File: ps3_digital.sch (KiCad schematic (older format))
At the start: 78 parts, among them SW2 SW_SPST, U1 SN75107B, U10 74LS08, U11 7425, U12 74LS32, U13 74LS193, U14 74LS153, U15 74LS74, U16 74LS93, U17 74LS244, U18 74LS367, U19 74LS367, U2 74LS175, U20 74LS32, U21 74LS74, U22 74LS266, U23 74LS266, U25 74LS08, U26 74LS08, U27 CD4051B, U28 74LS259, U29 74LS13, U3 74LS74, U30 74LS93, U31 74LS93, U32 74LS93, U33 74LS42, U34 74LS32, U35 74LS04, U36 7404, U37 4041, U38 4041, U39 TL072, U4 D2102, U40 TL082, U41 TL082, U42 TL082, U43 TL082, U44 L7805, U5 74LS00, U6 74LS04, U7 74LS10, U8 74LS00, U9 74LS32

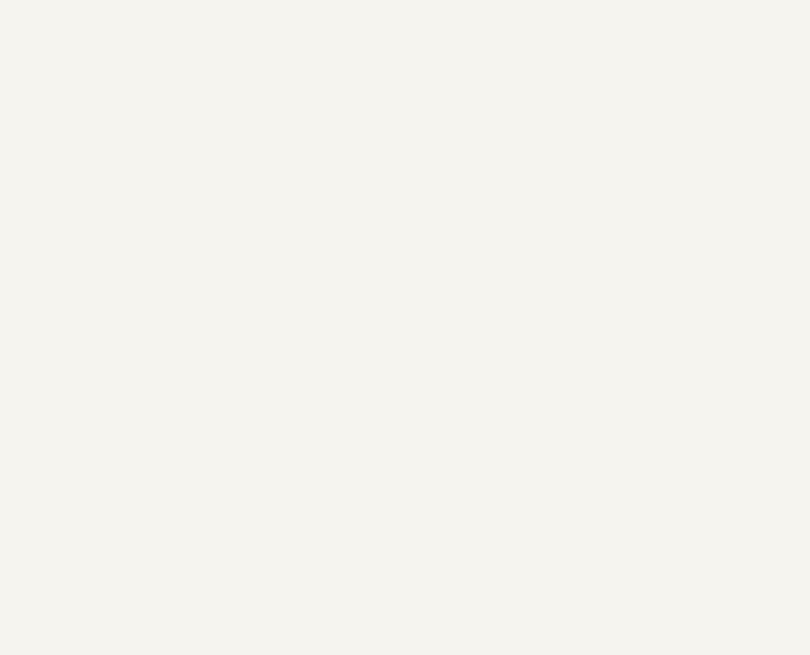
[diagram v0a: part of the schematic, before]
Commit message: 6810
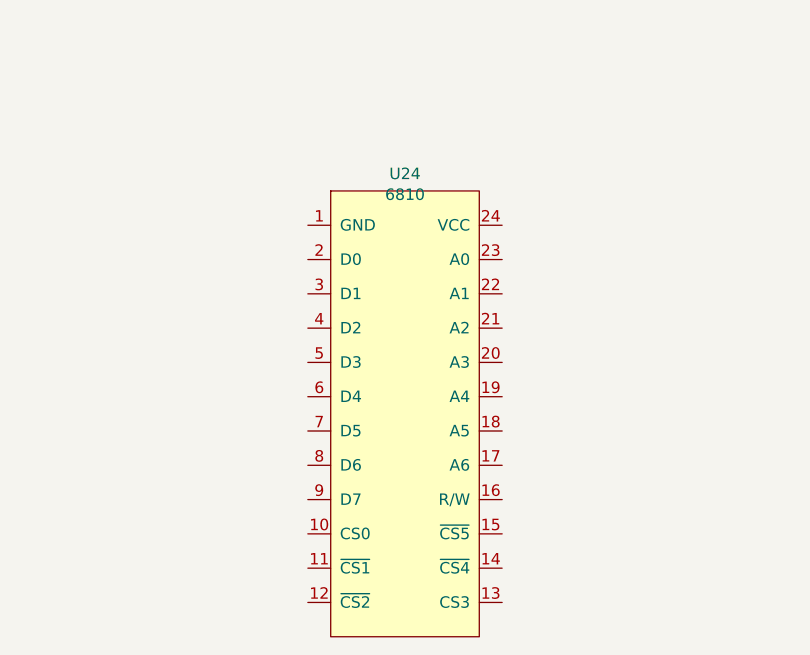
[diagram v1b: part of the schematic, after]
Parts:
- added U24: 6810, Package_DIP:DIP-24_W10.16mm_LongPads, symbol Memory_RAM:6810
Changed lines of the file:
@@
 	20250 6600 20500 6600
 Connection ~ 20250 6600
+$Comp
+L Memory_RAM:6810 U24
+U 1 1 5F25EB04
+P 13800 9700
+F 0 "U24" H 13775 10425 50  0000 C CNN
+F 1 "6810" H 13775 10334 50  0000 C CNN
+F 2 "Package_DIP:DIP-24_W10.16mm_LongPads" H 13800 9600 50  0001 C CNN
+F 3 "https://www.alldatasheet.com/datasheet-pdf/pdf/100353/MOTOROLA/MCM6810.html" H 13900 9600 50  0001 C CNN
+	1    13800 9700
+	1    0    0    -1
+$EndComp
 $EndSCHEMATC

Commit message: WIP
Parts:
- removed R20, R22: 200k, symbol Device:R
- removed unit 1 of U10
- removed unit 2 of U12
- removed unit 3 of U12
- removed unit 2 of U15
- removed unit 2 of U20
- removed unit 3 of U20
- removed unit 3 of U23
- removed unit 4 of U23
- removed unit 1 of U25
- removed unit 2 of U3
- removed unit 4 of U34
- removed unit 5 of U35
- removed unit 2 of U6
- removed unit 4 of U6
- removed unit 5 of U6
- removed unit 6 of U6
- removed unit 2 of U8
- added C10: 1nF, symbol Device:C_Small
- added C11: 22nF, symbol Device:C_Small
- added C12: 10uF, symbol Device:CP_Small
- added C13: 10Uf, symbol Device:CP_Small
- added C9: 4700uF, symbol Device:CP_Small
- added D1, D2, D3, D4: 1N4002, Diode_THT:D_DO-41_SOD81_P10.16mm_Horizontal, symbol Diode:1N4002
- added R10, R11, R9: 2k7, symbol Device:R
- added R6, R7, R8: 1k, symbol Device:R
- added SW1: SW_SP4T, symbol Switch:SW_SP4T
- gave numbers to parts that had none: 7
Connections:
- net Do is gone; now on net D0: U37.3
- net +15V: now also U39.8 (V+), U40.8 (V+), U41.8 (V+), U42.8 (V+), U43.8 (V+)
- net +5V: now also U10.14 (VCC), U11.11 (G), U11.3 (G), U12.14 (VCC), U13.11 (~LOAD), U13.16 (VCC), U14.16 (VCC), U15.14 (VCC), U15.2 (D), U15.4 (~S), U16.5 (VCC), U17.20 (VCC), U20.14 (VCC), U21.13 (~R), U21.14 (VCC), U24.10 (CS0), U24.13 (CS3), U24.24 (VCC), U25.14 (VCC), U26.14 (VCC), U28.15 (Clr), U28.16 (VCC), U29.14 (VCC), U3.14 (VCC), U30.5 (VCC), U31.5 (VCC), U32.5 (VCC), U33.16 (VCC), U34.14 (VCC), U35.14 (VCC), U44.3 (OUT), U5.14 (VCC), U6.14 (VCC), U7.1, U7.14 (VCC), U7.2, U8.14 (VCC), U9.14 (VCC), C13.1, R10.1, R11.1, R6.1, R9.1; no longer U21.12 (D)
- net A0: now also U22.8, U31.9 (Q1), U36.1
- net A1: now also U31.8 (Q2), U36.3
- net A2: now also U31.11 (Q3), U32.14 (CP0), U36.5, U8.10; no longer U19.5 (O2a)
- net A3: now also U18.2 (I1), U32.1 (CP1..3), U32.12 (Q0), U36.9
- net A4: now also U18.4 (I2), U32.9 (Q1), U36.11
- net A5: now also U18.6 (I3), U32.8 (Q2), U36.13; no longer U19.7 (O3a)
- net D0: now also U24.2 (D0)
- net D1: now also U22.13, U24.3 (D1)
- net D2: now also U19.5 (O2a), U22.1, U24.4 (D2)
- net D3: now also U22.5, U24.5 (D3)
- net D4: now also U23.2, U24.6 (D4)
- net D5: now also U19.7 (O3a), U23.5, U24.7 (D5)
- net GND: now also U10.7 (GND), U11.12, U11.13, U12.7 (GND), U13.8 (GND), U14.1 (Ea), U14.3 (I3a), U14.8 (GND), U15.7 (GND), U16.10 (GND), U17.10 (GND), U20.7 (GND), U21.7 (GND), U24.1 (GND), U24.11 (~CS1), U24.12 (~CS2), U24.14 (~CS4), U24.15 (~CS5), U24.17 (A6), U24.18 (A5), U24.19 (A4), U24.20 (A3), U25.7 (GND), U26.7 (GND), U28.8 (GND), U29.7 (GND), U3.7 (GND), U30.10 (GND), U30.2 (R0(1)), U30.3 (R0(2)), U31.10 (GND), U31.2 (R0(1)), U31.3 (R0(2)), U32.10 (GND), U32.2 (R0(1)), U32.3 (R0(2)), U33.8 (GND), U34.7 (GND), U35.7 (GND), U5.7 (GND), U6.7 (GND), U7.7 (GND), U8.7 (GND), U9.7 (GND), C10.2, R7.2, SW1.3
- net IC2-D3: now also U5.11
- net ~ANC: now also U20.13
- net ~CLC: now also U20.1
- net ~CP1: now also U21.11 (C), U21.3 (C), U33.2 (1)
- net ~F2: now also U35.2
- net ~KU: now also U35.5
- net ~RW: now also U34.8, U9.4
- net IC2_11: now reaches U2.11 (~Q2)
- net IC2_11: now also U7.11, U7.4, U8.12
- net at U15.1 (~R): now also U35.6
- net ~M: now reaches U15.3 (C)
- net ~M: now also U35.12, C11.2
- net at U15.6 (~Q): now also U11.10
- net at R5.2, U21.2 (D), U22.10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: now also U22.4
- net at U21.9 (Q): now also U7.5
- net at U8.3: now also U12.2, U9.9
- net at U8.8: now also U27.6 (INH), U28.14 (E)
- net M: now reaches U8.9
- net M: now also U18.1 (OEa), U20.12, U20.2, U32.11 (Q3), U33.13 (A2), U35.13
- net at U8.13: now also U7.12, U7.3
- net F2: now reaches U35.1
- net F2: now also U17.11 (I0b), U29.10, U29.9, U31.1 (CP1..3), U31.12 (Q0)
- net CK0: now reaches U35.3
- net CK0: now also U29.6, U30.14 (CP0), R8.1
- net at U35.4: now also U33.12 (A3)
- net at U35.8: now also U34.5
- net at U35.9: now also U29.8, U34.2, U34.9
- net at U7.13: now also U12.12, U14.9 (Zb), U7.10
- net at U7.6: now also U9.1
- net ~CP3: now reaches U9.2
- net ~CP3: now also U34.6
- net at U9.3: now also U10.13
- net at U9.5: now also U10.6, U9.12
- net at U9.6: now also U10.9
- net ~CP2: now reaches U9.10
- net ~CP2: now also U33.3 (2), U34.10, U34.4
- net at U9.8: now also U10.10
- net ~TGU: now reaches U9.11
- net ~TGU: now also U10.12, U12.13
- net ~UC: now reaches U9.13
- net ~UC: now also U34.3
- net at U12.1: now also U11.6
- net at U12.3: now also U13.4 (DOWN)
- net at U20.3: now also U17.1 (OEa)
- net at U34.1: now also U33.4 (3)
- net at U12.11: now also U13.5 (UP)
- net at U20.11: now also U17.19 (OEb)
- net at U10.8: now also U18.15 (OEb), U19.1 (OEa), U19.15 (OEb), U24.16 (R/W)
- net at U10.11: now also U16.1 (CP1..3)
- net IC18_3: now reaches U25.4
- net IC18_3: now also U17.16 (O1a), U17.5 (O2b), U18.3 (O1a), U27.11 (A), U28.1 (A0)
- net 1: now reaches U25.5
- net 1: now also U26.1, U26.13, U26.9, R9.2, SW1.1
- net at U25.6: now also U24.23 (A0)
- net IC18_5: now reaches U25.10
- net IC18_5: now also U17.14 (O2a), U17.7 (O1b), U18.5 (O2a), U27.10 (B), U28.2 (A1)
- net at U25.8: now also U24.22 (A1)
- net at U25.9: now also U26.3, U26.4
- net at U25.11: now also U24.21 (A2)
- net at U25.12: now also U26.6
- net IC18_7: now reaches U25.13
- net IC18_7: now also U17.12 (O3a), U17.9 (O0b), U18.7 (O3a), U27.9 (C), U28.3 (A2)
- net 2: now reaches U26.2
- net 2: now also U26.10, R10.2, SW1.2
- net 4: now reaches U26.5
- net 4: now also U26.12, R11.2, SW1.4
- net SL1: now reaches U26.8
- net SL1: now also U14.2 (S1)
- net SL2: now reaches U26.11
- net SL2: now also U14.14 (S0)
- net at U11.1: now also U13.3 (QA), U14.10 (I0b)
- net at U11.2: now also U13.2 (QB), U14.11 (I1b)
- net at U11.4: now also U13.6 (QC), U14.12 (I2b)
- net at U11.5: now also U13.7 (QD), U14.13 (I3b)
- net at U11.8: now also U13.14 (CLR)
- net at U11.9: now also C11.1, R6.2, R7.1
- net IC14_4: now reaches U14.4 (I2a)
- net IC14_4: now also U16.11 (Q3), U17.8 (I3a)
- net IC14_5: now reaches U14.5 (I1a)
- net IC14_5: now also U16.8 (Q2), U17.6 (I2a)
- net IC14_6: now reaches U14.6 (I0a)
- net IC14_6: now also U16.9 (Q1), U17.4 (I1a)
- net IC14_7: now reaches U14.7 (Za)
- net IC14_7: now also U16.2 (R0(1)), U16.3 (R0(2))
- net CK1: now reaches U30.1 (CP1..3)
- net CK1: now also U30.12 (Q0), U33.15 (A0)
- net F1: now reaches U30.11 (Q3)
- net F1: now also U17.13 (I1b), U29.12, U31.14 (CP0)
- net F0: now reaches U30.8 (Q2)
- net F0: now also U17.15 (I2b), U29.13
- net CK2: now reaches U30.9 (Q1)
- net CK2: now also U33.14 (A1)
- net at U18.11 (O5b): now also U21.12 (D), U24.8 (D6), U28.13 (D)
- net G6: now reaches U28.10 (Q5)
- net G7: now reaches U28.11 (Q6)
- net G8: now reaches U28.12 (Q7)
- net G1: now reaches U28.4 (Q0)
- net G2: now reaches U28.5 (Q1)
- net G3: now reaches U28.6 (Q2)
- net G4: now reaches U28.7 (Q3)
- net G5: now reaches U28.9 (Q4)
- net at U29.1: now also U29.2, U29.4, U29.5, C10.1, R8.2
- net K0: now reaches U36.2
- net K1: now reaches U36.4
- net K2: now reaches U36.6
- net K3: now reaches U36.8
- net K4: now reaches U36.10
- net K5: now reaches U36.12
- net -15V: now reaches U40.4 (V-)
- net -15V: now also U39.4 (V-), U41.4 (V-), U42.4 (V-), U43.4 (V-)
- net at U44.1 (IN): now also C12.1, C9.1, D3.1 (K), D4.2 (A)
- net GNDD: now reaches U44.2 (GND)
- net GNDD: now also C12.2, C13.2, C9.2, D1.2 (A), D4.1 (K)
- new net: D2.1 (K), D3.2 (A)
- new net: D1.1 (K), D2.2 (A)
- new net 8: SW1.5
- no-connect marks 0 -> 8
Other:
- note added: "GATE OUTPUTS"
- note added: "KEYBOARD ADDRESS BUFFER"
- note added: "NO. OF VOICES"
- note added: "New note priority"
- note added: "PITH VOLTAGE\nOUTPUTS\n(TO PORTAMENTO UNITS)"
- moved on the sheet: C25, C26, C27, R12, R13, R14, R15, R16, R17, R18, R19, R20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
